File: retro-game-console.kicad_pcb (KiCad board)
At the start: 2 copper layers, 96.5 x 137.2 mm, 42 parts, among them J1 Battery_Clip, U1 ESP32-DevKitC, U2 Battery_shield_v3, U3 Micro_SD_card_adapter, U4 MAX98357A_Breakout, U5 LCD_ILI9341, U6 74HC165

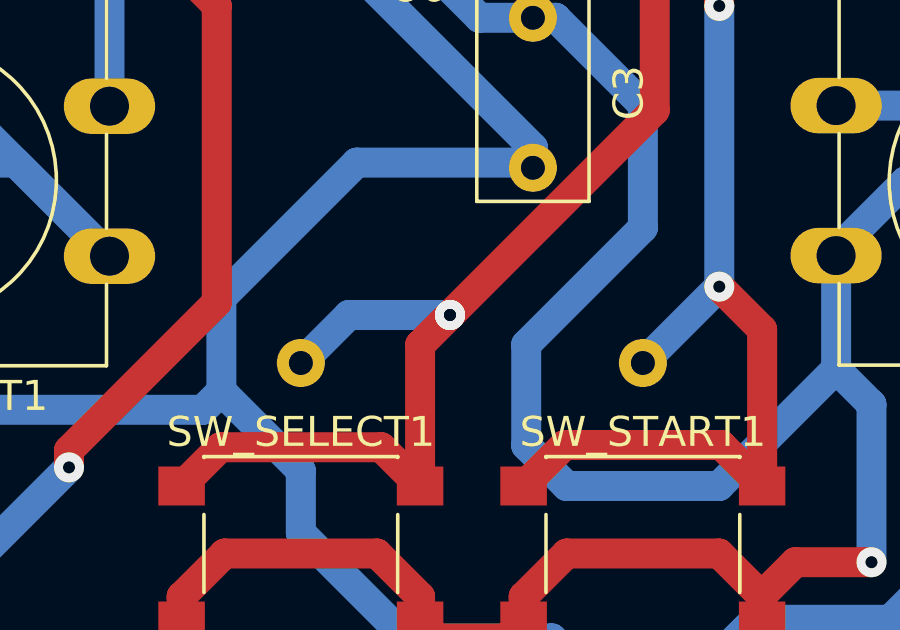
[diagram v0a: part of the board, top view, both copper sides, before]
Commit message: snapshot
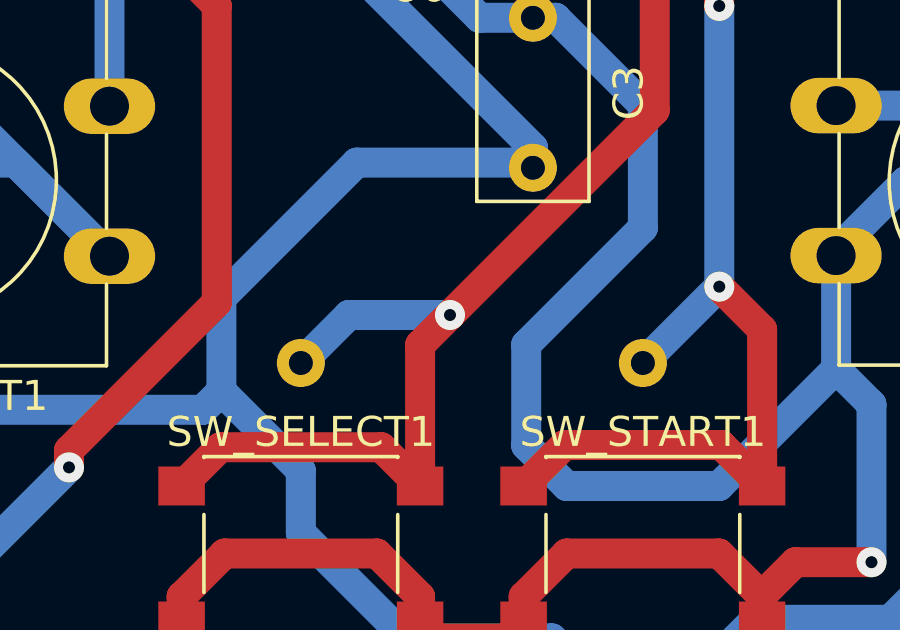
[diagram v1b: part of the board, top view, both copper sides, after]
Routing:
- net BTN_SELECT: vias 3 -> 2
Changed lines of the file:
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@@
   (segment (start 67.784514 125.255486) (end 67.784514 114.920261) (width 1) (layer "F.Cu") (net 26))
   (segment (start 52.012772 137.780261) (end 53.304908 136.488125) (width 1) (layer "F.Cu") (net 26))
-  (via (at 60.96 132.08) (size 1) (drill 0.4) (layers "F.Cu" "B.Cu") (net 26))
   (via (at 67.784514 114.920261) (size 1) (drill 0.4) (layers "F.Cu" "B.Cu") (net 26))
   (via (at 60.96 132.08) (size 1) (drill 0.4) (layers "F.Cu" "B.Cu") (net 26))
